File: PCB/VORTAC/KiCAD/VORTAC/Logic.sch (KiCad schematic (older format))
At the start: 61 parts, among them Q1 Q_PMOS_GSD, Q2 Q_NMOS_GSD, Q3 WSD4066DN, Q4 Q_NMOS_GSD, Q5 WSD4066DN, Q6 Q_PNP_BEC, Q7 Q_NPN_BEC, U1 TLV73333PDBV, U3 TPS54335ADRCR, U4 TPS54335ADRCR

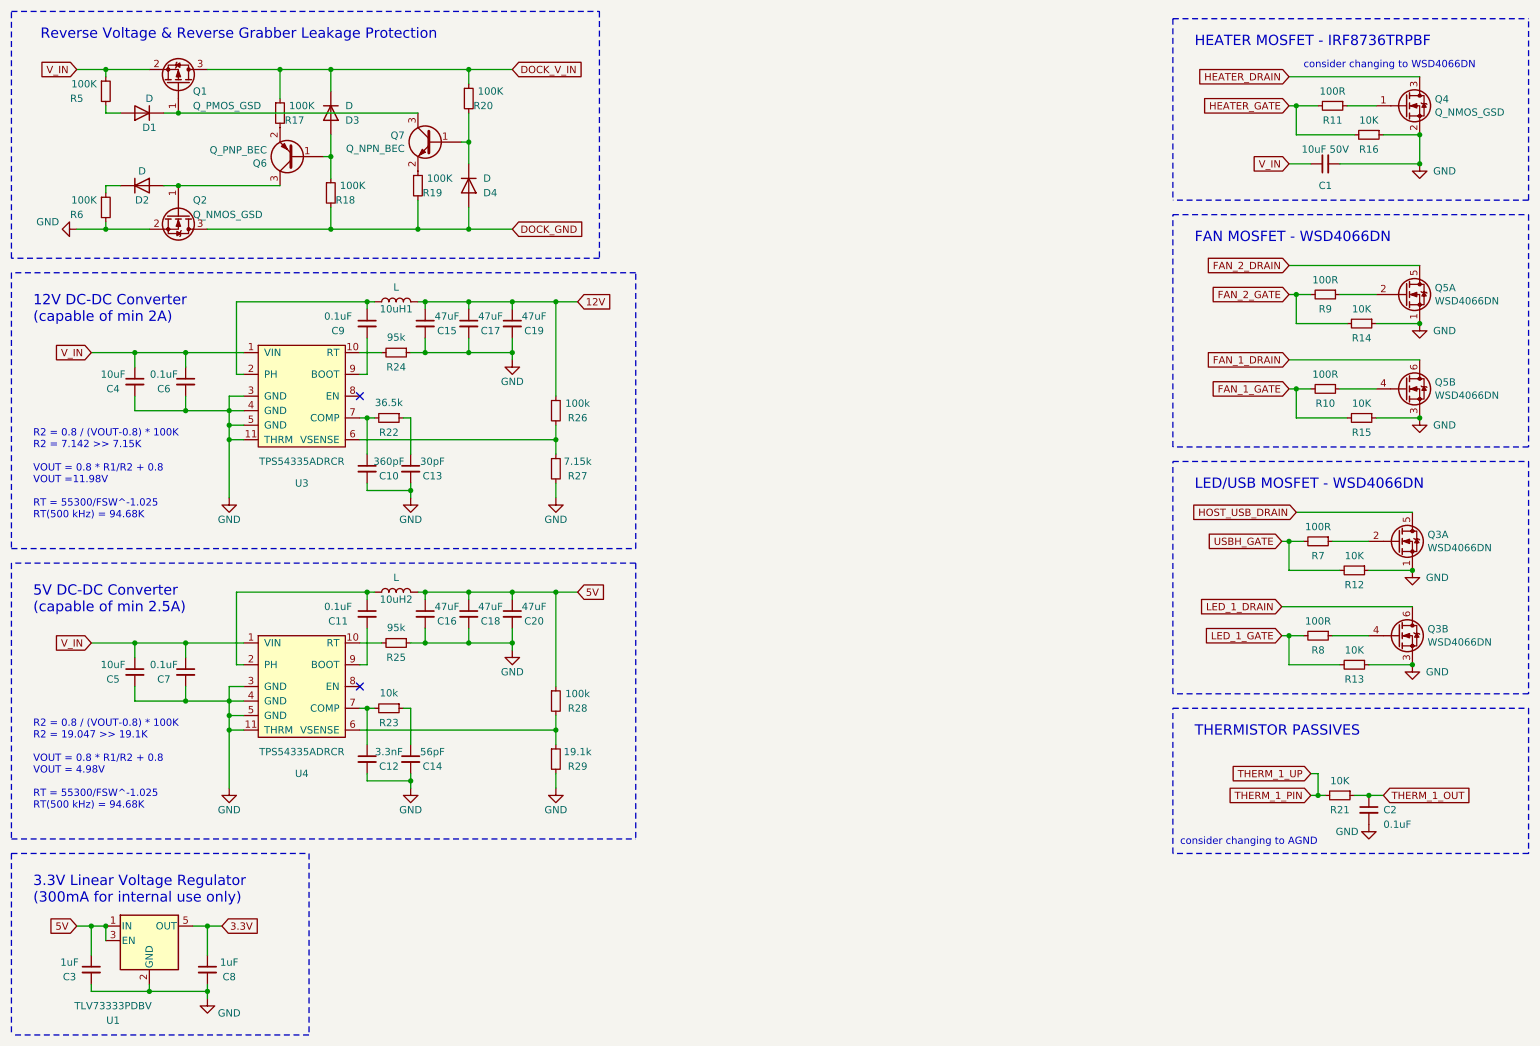
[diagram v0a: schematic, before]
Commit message: Routing WIP
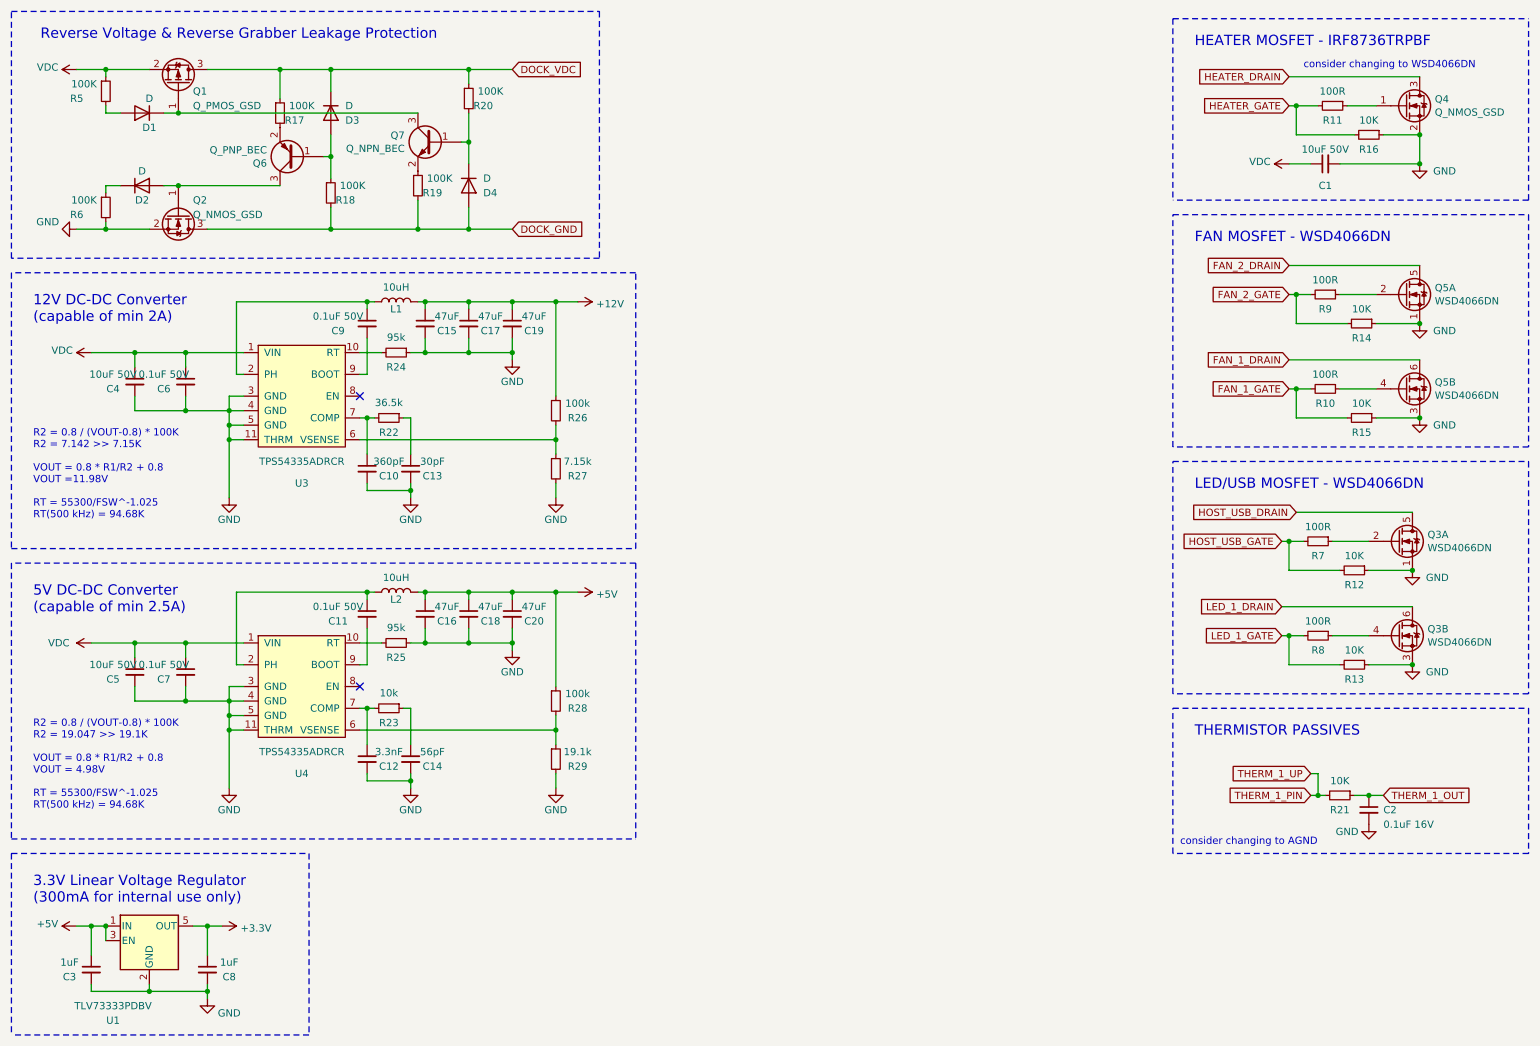
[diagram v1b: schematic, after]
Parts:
- C1: footprint Resistor_SMD:R_0603_1608Metric -> Capacitor_SMD:C_1206_3216Metric; LCSC (none) -> C89632
- C11, C6, C7, C9: value 0.1uF -> 0.1uF 50V
- C2: value 0.1uF -> 0.1uF 16V; footprint Capacitor_SMD:C_0402_1005Metric -> Capacitor_SMD:C_0603_1608Metric; LCSC (none) -> C66501
- C3, C8: LCSC C152910 -> (none)
- C4, C5: value 10uF -> 10uF 50V
- L1: renamed from 10uH1; value L -> 10uH
- L2: renamed from 10uH2; value L -> 10uH
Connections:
- net 12V renamed +12V
- net 3.3V renamed +3V3
- net 5V renamed +5V
- net DOCK_V_IN renamed DOCK_VDC
- net USBH_GATE renamed HOST_USB_GATE
- net V_IN renamed VDC
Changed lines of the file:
@@
 HOST_USB_DRAIN
 Text GLabel 9350 4250 0    50   Input ~ 0
-USBH_GATE
+HOST_USB_GATE
 Text GLabel 9350 4900 0    50   Input ~ 0
 LED_1_GATE
@@
 Text GLabel 9400 1050 0    50   Input ~ 0
 HEATER_DRAIN
-Text GLabel 9400 1650 0    50   Input ~ 0
-V_IN
 $Comp
 L Device:Q_NMOS_GSD Q4
@@
 F 0 "C1" V 9500 1650 50  0000 C CNN
 F 1 "10uF 50V" V 9750 1650 50  0000 C CNN
-F 2 "Resistor_SMD:R_0603_1608Metric" H 9650 1650 50  0001 C CNN
-F 3 "~" H 9650 1650 50  0001 C CNN
+F 2 "Capacitor_SMD:C_1206_3216Metric" H 9650 1650 50  0001 C CNN
+F 3 "https://www.lcsc.com/product-detail/Multilayer-Ceramic-Capacitors-MLCC-SMD-SMT_Samsung-Electro-Mechanics-CL31B106KBHNNNE_C89632.html" H 9650 1650 50  0001 C CNN
+F 4 "C89632" H 9650 1650 50  0001 C CNN "LCSC"
 	1    9650 1650
 	0    -1   -1   0
@@
 Connection ~ 10300 1650
 Text GLabel 4050 1000 2    50   Input ~ 0
-DOCK_V_IN
+DOCK_VDC
 Text GLabel 4050 2100 2    50   Input ~ 0
 DOCK_GND
@@
 	0    1    1    0
 $EndComp
-Text GLabel 1050 1000 0    50   Input ~ 0
-V_IN
 $Comp
 L Device:D D1
@@
 AR Path="/613DB78D/6170C67D" Ref="C?"  Part="1"
 F 0 "C2" H 10050 6100 50  0000 L CNN
-F 1 "0.1uF" H 10050 6000 50  0000 L CNN
-F 2 "Capacitor_SMD:C_0402_1005Metric" H 9950 6100 50  0001 C CNN
-F 3 "~" H 9950 6100 50  0001 C CNN
+F 1 "0.1uF 16V" H 10050 6000 50  0000 L CNN
+F 2 "Capacitor_SMD:C_0603_1608Metric" H 9950 6100 50  0001 C CNN
+F 3 "https://www.lcsc.com/product-detail/Multilayer-Ceramic-Capacitors-MLCC-SMD-SMT_Samsung-Electro-Mechanics-CL10B104KO8NNNC_C66501.html" H 9950 6100 50  0001 C CNN
+F 4 "C66501" H 9950 6100 50  0001 C CNN "LCSC"
 	1    9950 6100
 	1    0    0    -1
@@
 AR Path="/613DC005/63288FE5" Ref="C?"  Part="1"
 F 0 "C9" H 2850 2700 50  0000 C CNN
-F 1 "0.1uF" H 2850 2800 50  0000 C CNN
+F 1 "0.1uF 50V" H 2850 2800 50  0000 C CNN
 F 2 "Capacitor_SMD:C_0603_1608Metric" H 3050 2750 50  0001 C CNN
 F 3 "https://www.lcsc.com/product-detail/Multilayer-Ceramic-Capacitors-MLCC-SMD-SMT_Samsung-Electro-Mechanics-CL10B104KB8NNNC_C1591.html" H 3050 2750 50  0001 C CNN
@@
 Wire Wire Line
 	2150 3100 2200 3100
-Text GLabel 1150 2950 0    50   Input ~ 0
-V_IN
 $Comp
 L Device:C_Small C4
@@
 AR Path="/613DC005/63289031" Ref="C?"  Part="1"
 F 0 "C4" H 1300 3100 50  0000 C CNN
-F 1 "10uF" H 1300 3200 50  0000 C CNN
+F 1 "10uF 50V" H 1300 3200 50  0000 C CNN
 F 2 "Capacitor_SMD:C_1206_3216Metric" H 1450 3150 50  0001 C CNN
 F 3 "https://www.lcsc.com/product-detail/Multilayer-Ceramic-Capacitors-MLCC-SMD-SMT_Samsung-Electro-Mechanics-CL31B106KBHNNNE_C89632.html" H 1450 3150 50  0001 C CNN
@@
 AR Path="/613DC005/63289038" Ref="C?"  Part="1"
 F 0 "C6" H 1650 3100 50  0000 C CNN
-F 1 "0.1uF" H 1650 3200 50  0000 C CNN
+F 1 "0.1uF 50V" H 1650 3200 50  0000 C CNN
 F 2 "Capacitor_SMD:C_0603_1608Metric" H 1800 3150 50  0001 C CNN
 F 3 "https://www.lcsc.com/product-detail/Multilayer-Ceramic-Capacitors-MLCC-SMD-SMT_Samsung-Electro-Mechanics-CL10B104KB8NNNC_C1591.html" H 1800 3150 50  0001 C CNN
@@
 AR Path="/613DC005/63289050" Ref="C?"  Part="1"
 F 0 "C11" H 2850 4700 50  0000 C CNN
-F 1 "0.1uF" H 2850 4800 50  0000 C CNN
+F 1 "0.1uF 50V" H 2850 4800 50  0000 C CNN
 F 2 "Capacitor_SMD:C_0603_1608Metric" H 3050 4750 50  0001 C CNN
 F 3 "https://www.lcsc.com/product-detail/Multilayer-Ceramic-Capacitors-MLCC-SMD-SMT_Samsung-Electro-Mechanics-CL10B104KB8NNNC_C1591.html" H 3050 4750 50  0001 C CNN
@@
 P 3250 4600
 AR Path="/613DC005/6328905D" Ref="10uH?"  Part="1"
-AR Path="/613DBE83/6328905D" Ref="10uH2"  Part="1"
-F 0 "10uH2" V 3200 4600 50  0000 C CNN
-F 1 "L" V 3350 4600 50  0000 C CNN
+AR Path="/613DBE83/6328905D" Ref="L2"  Part="1"
+F 0 "L2" V 3200 4600 50  0000 C CNN
+F 1 "10uH" V 3350 4600 50  0000 C CNN
 F 2 "ToolChanger:L_Sunlord_MWSA0518_5.4x5.2mm" H 3250 4600 50  0001 C CNN
 F 3 "https://www.lcsc.com/product-detail/Power-Inductors_Sunlord-MWSA0503S-100MT_C408412.html" H 3250 4600 50  0001 C CNN
@@
 Wire Wire Line
 	3050 5900 3350 5900
-Text GLabel 4500 4600 2    50   Input ~ 0
-5V
 Wire Wire Line
 	4350 4600 4500 4600
@@
 Wire Wire Line
 	2150 5100 2200 5100
-Text GLabel 1150 4950 0    50   Input ~ 0
-V_IN
 $Comp
 L Device:C_Small C5
@@
 AR Path="/613DC005/632890DF" Ref="C?"  Part="1"
 F 0 "C5" H 1300 5100 50  0000 C CNN
-F 1 "10uF" H 1300 5200 50  0000 C CNN
+F 1 "10uF 50V" H 1300 5200 50  0000 C CNN
 F 2 "Capacitor_SMD:C_1206_3216Metric" H 1450 5150 50  0001 C CNN
 F 3 "https://www.lcsc.com/product-detail/Multilayer-Ceramic-Capacitors-MLCC-SMD-SMT_Samsung-Electro-Mechanics-CL31B106KBHNNNE_C89632.html" H 1450 5150 50  0001 C CNN
@@
 AR Path="/613DC005/632890E6" Ref="C?"  Part="1"
 F 0 "C7" H 1650 5100 50  0000 C CNN
-F 1 "0.1uF" H 1650 5200 50  0000 C CNN
+F 1 "0.1uF 50V" H 1650 5200 50  0000 C CNN
 F 2 "Capacitor_SMD:C_0603_1608Metric" H 1800 5150 50  0001 C CNN
 F 3 "https://www.lcsc.com/product-detail/Multilayer-Ceramic-Capacitors-MLCC-SMD-SMT_Samsung-Electro-Mechanics-CL10B104KB8NNNC_C1591.html" H 1800 5150 50  0001 C CNN
@@
 Wire Wire Line
 	4350 2600 4500 2600
-Text GLabel 4500 2600 2    50   Input ~ 0
-12V
 Connection ~ 3750 2950
 Wire Wire Line
@@
 P 3250 2600
 AR Path="/613DC005/6328913B" Ref="10uH?"  Part="1"
-AR Path="/613DBE83/6328913B" Ref="10uH1"  Part="1"
-F 0 "10uH1" V 3200 2600 50  0000 C CNN
-F 1 "L" V 3350 2600 50  0000 C CNN
+AR Path="/613DBE83/6328913B" Ref="L1"  Part="1"
+F 0 "L1" V 3200 2600 50  0000 C CNN
+F 1 "10uH" V 3350 2600 50  0000 C CNN
 F 2 "ToolChanger:L_Sunlord_MWSA0518_5.4x5.2mm" H 3250 2600 50  0001 C CNN
 F 3 "https://www.lcsc.com/product-detail/Power-Inductors_Sunlord-MWSA0503S-100MT_C408412.html" H 3250 2600 50  0001 C CNN
@@
 	1    0    0    -1
 $EndComp
-Text GLabel 1050 6900 0    50   Input ~ 0
-5V
-Text GLabel 2050 6900 2    50   Input ~ 0
-3.3V
 $Comp
 L Device:C_Small C8
@@
 F 1 "1uF" H 2100 7250 50  0000 C CNN
 F 2 "Capacitor_SMD:C_0603_1608Metric" H 1950 7200 50  0001 C CNN
-F 3 "https://www.lcsc.com/product-detail/Multilayer-Ceramic-Capacitors-MLCC-SMD-SMT_Walsin-Tech-Corp-0603N332J500CT_C152910.html" H 1950 7200 50  0001 C CNN
-F 4 "C152910" H 1950 7200 50  0001 C CNN "LCSC"
+F 3 "" H 1950 7200 50  0001 C CNN
+F 4 "" H 1950 7200 50  0001 C CNN "LCSC"
 	1    1950 7200
 	1    0    0    -1
@@
 F 1 "1uF" H 1000 7250 50  0000 C CNN
 F 2 "Capacitor_SMD:C_0603_1608Metric" H 1150 7200 50  0001 C CNN
-F 3 "https://www.lcsc.com/product-detail/Multilayer-Ceramic-Capacitors-MLCC-SMD-SMT_Walsin-Tech-Corp-0603N332J500CT_C152910.html" H 1150 7200 50  0001 C CNN
-F 4 "C152910" H 1150 7200 50  0001 C CNN "LCSC"
+F 3 "" H 1150 7200 50  0001 C CNN
+F 4 "" H 1150 7200 50  0001 C CNN "LCSC"
 	1    1150 7200
 	1    0    0    -1
@@
 Wire Wire Line
 	9450 4050 10250 4050
+$Comp
+L power:VDC #PWR0140
+U 1 1 61FDF6CF
+P 9400 1650
+F 0 "#PWR0140" H 9400 1550 50  0001 C CNN
+F 1 "VDC" V 9415 1777 50  0000 L CNN
+F 2 "" H 9400 1650 50  0001 C CNN
+F 3 "" H 9400 1650 50  0001 C CNN
+	1    9400 1650
+	0    -1   -1   0
+$EndComp
+$Comp
+L power:VDC #PWR0141
+U 1 1 620077AC
+P 1050 1000
+F 0 "#PWR0141" H 1050 900 50  0001 C CNN
+F 1 "VDC" V 1065 1127 50  0000 L CNN
+F 2 "" H 1050 1000 50  0001 C CNN
+F 3 "" H 1050 1000 50  0001 C CNN
+	1    1050 1000
+	0    -1   -1   0
+$EndComp
+$Comp
+L power:VDC #PWR0142
+U 1 1 62013F8B
+P 1150 2950
+F 0 "#PWR0142" H 1150 2850 50  0001 C CNN
+F 1 "VDC" V 1165 3077 50  0000 L CNN
+F 2 "" H 1150 2950 50  0001 C CNN
+F 3 "" H 1150 2950 50  0001 C CNN
+	1    1150 2950
+	0    -1   -1   0
+$EndComp
+$Comp
+L power:VDC #PWR0143
+U 1 1 62022D6D
+P 1150 4950
+F 0 "#PWR0143" H 1150 4850 50  0001 C CNN
+F 1 "VDC" V 1150 5100 50  0000 L CNN
+F 2 "" H 1150 4950 50  0001 C CNN
+F 3 "" H 1150 4950 50  0001 C CNN
+	1    1150 4950
+	0    -1   -1   0
+$EndComp
+$Comp
+L power:+5V #PWR0144
+U 1 1 6203746B
+P 1050 6900
+F 0 "#PWR0144" H 1050 6750 50  0001 C CNN
+F 1 "+5V" V 1065 7028 50  0000 L CNN
+F 2 "" H 1050 6900 50  0001 C CNN
+F 3 "" H 1050 6900 50  0001 C CNN
+	1    1050 6900
+	0    -1   -1   0
+$EndComp
+$Comp
+L power:+3.3V #PWR0145
+U 1 1 62038159
+P 2050 6900
+F 0 "#PWR0145" H 2050 6750 50  0001 C CNN
+F 1 "+3.3V" V 2065 7028 50  0000 L CNN
+F 2 "" H 2050 6900 50  0001 C CNN
+F 3 "" H 2050 6900 50  0001 C CNN
+	1    2050 6900
+	0    1    1    0
+$EndComp
+$Comp
+L power:+5V #PWR0146
+U 1 1 6203A774
+P 4500 4600
+F 0 "#PWR0146" H 4500 4450 50  0001 C CNN
+F 1 "+5V" V 4515 4728 50  0000 L CNN
+F 2 "" H 4500 4600 50  0001 C CNN
+F 3 "" H 4500 4600 50  0001 C CNN
+	1    4500 4600
+	0    1    1    0
+$EndComp
+$Comp
+L power:+12V #PWR0147
+U 1 1 62048089
+P 4500 2600
+F 0 "#PWR0147" H 4500 2450 50  0001 C CNN
+F 1 "+12V" V 4515 2728 50  0000 L CNN
+F 2 "" H 4500 2600 50  0001 C CNN
+F 3 "" H 4500 2600 50  0001 C CNN
+	1    4500 2600
+	0    1    1    0
+$EndComp
 $EndSCHEMATC
